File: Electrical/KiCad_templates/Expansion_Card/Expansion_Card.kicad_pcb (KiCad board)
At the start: 2 copper layers, 26 x 30 mm, 11 parts, among them P1 USB_C_Plug_USB2.0, U1 AP2112K-3.3

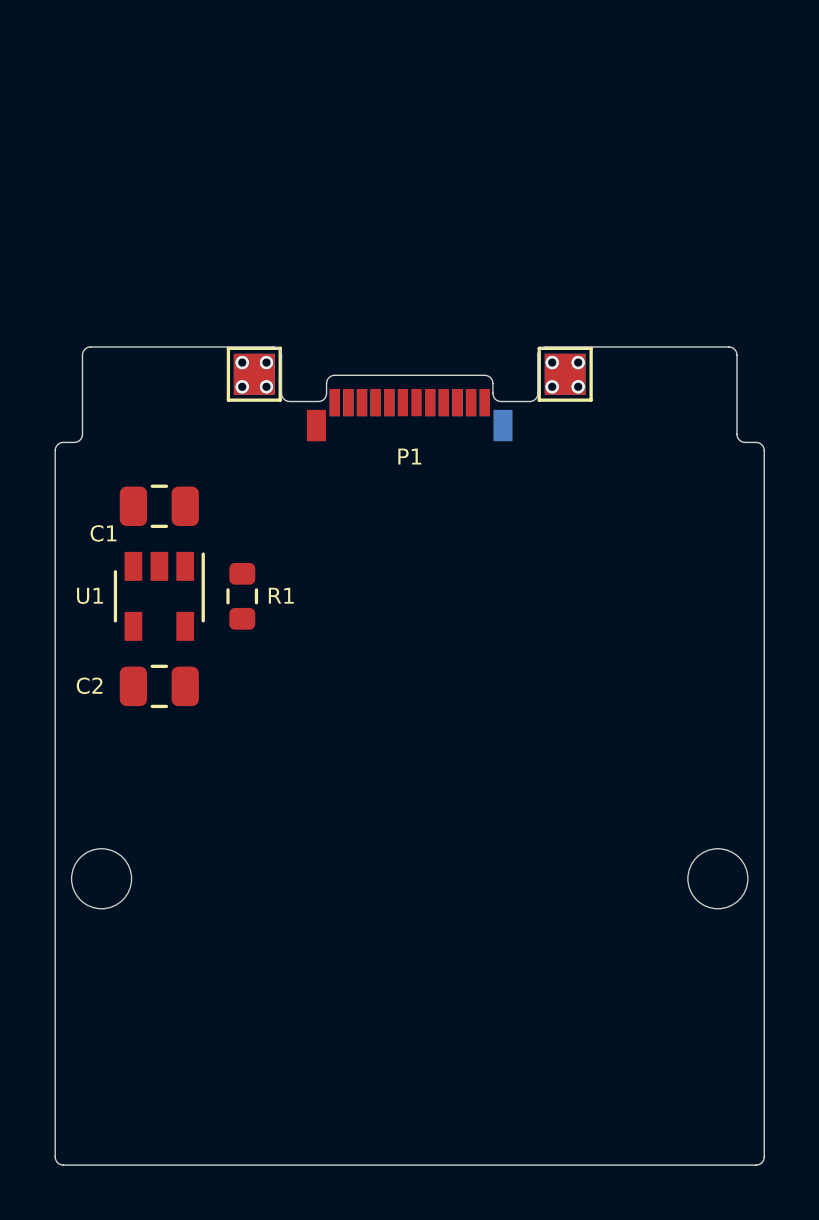
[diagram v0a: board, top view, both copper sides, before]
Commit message: Submitted for fabrication
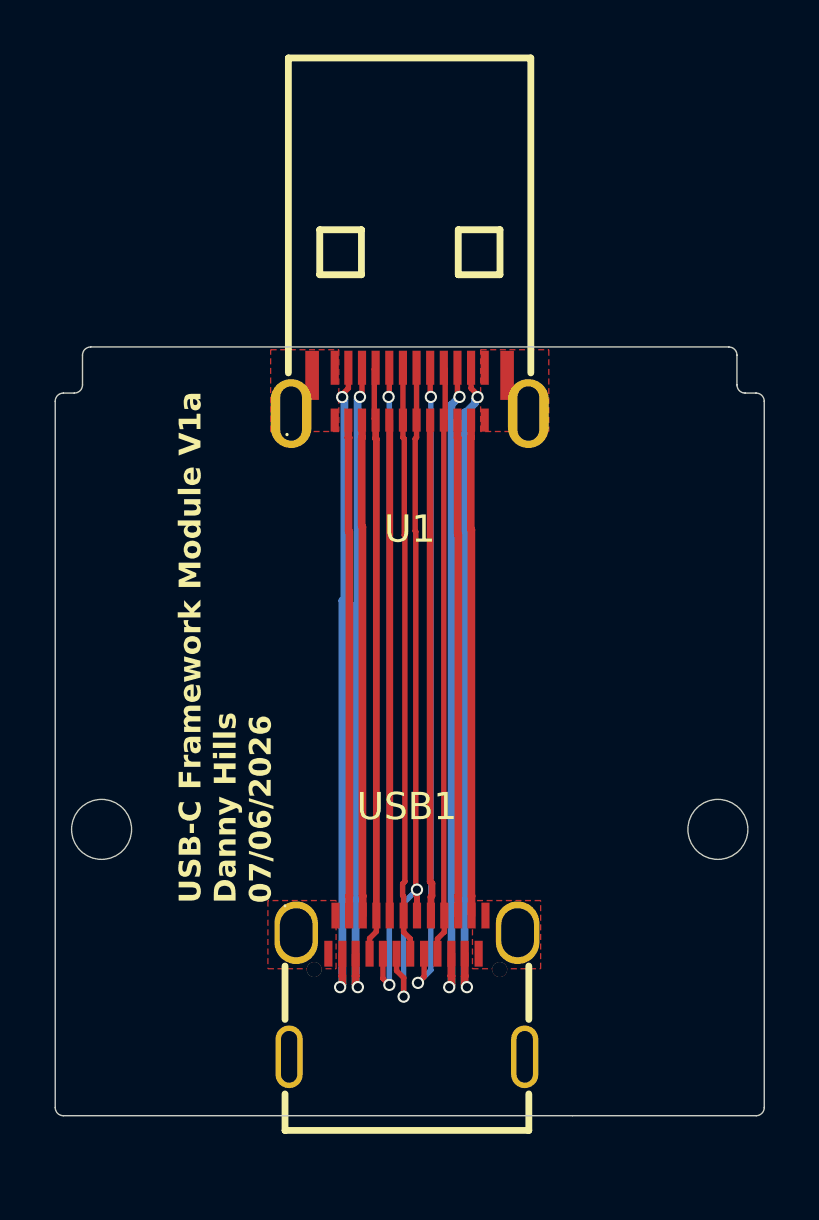
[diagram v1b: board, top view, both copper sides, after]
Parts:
- removed C1, C2: 10uF, Capacitor_SMD:C_0805_2012Metric
- removed P1: USB_C_Plug_USB2.0, Expansion_Card:USB_C_Plug_Molex_105444
- removed R1: 5.1k, Resistor_SMD:R_0603_1608Metric
- removed TP1, TP2, TP3, TP4: TestPoint, TestPoint:TestPoint_Pad_1.5x1.5mm
- added USB1: TYPE-C 24P QT 143, easyeda2kicad:TYPE-C-SMD_C9900025773, F.Cu at (139.9, 150.4)
- U1: value AP2112K-3.3 -> U261-241N-4BC2SS; footprint Package_TO_SOT_SMD:SOT-23-5 -> easyeda2kicad:USB-C-SMD_XKB_U261-24XN-4BC2SS
- moved U1 11.8 mm to (140.0, 128.7), turned to 180 degrees
- moved H1 1.81 mm to (128.7, 144.7)
- moved H2 1.81 mm to (151.3, 144.7)
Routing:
- net VBUS: track 0.00 -> 43.3 mm
- net /USB_DN: track 0.00 -> 26.9 mm, vias 0 -> 2
- net /RX2+: track 0.00 -> 24.3 mm, vias 0 -> 2
- net /RX2-: track 0.00 -> 24.2 mm, vias 0 -> 2
- net /TX1+: track 0.00 -> 24.2 mm, vias 0 -> 2
- net /TX1-: track 0.00 -> 24.1 mm, vias 0 -> 2
- net /SBU1: track 0.00 -> 23.9 mm, vias 0 -> 2
- net /CC: track 0.00 -> 23.9 mm, vias 0 -> 2
- net /USB_DP: track 0.00 -> 21.7 mm
- net /Vconn: track 0.00 -> 18.2 mm
- net /RX1+: track 0.00 -> 18.2 mm
- net /RX1-: track 0.00 -> 18.2 mm
- net /TX2-: track 0.00 -> 18.2 mm
- net /TX2+: track 0.00 -> 18.2 mm
- net /SBU2: track 0.00 -> 18.2 mm
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- added copper zone on F.Cu, net GND
- added copper zone on In1.Cu, net GND
- added copper zone on In2.Cu, net GND
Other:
- board size 26 x 30 mm -> 26 x 28.2 mm
- copper layers 2 -> 4
- net class Default removed
- board text added: "USB-C Framework Module V1a Danny Hills 07/06/2026"
